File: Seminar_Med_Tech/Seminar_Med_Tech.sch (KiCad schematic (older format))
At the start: 25 parts

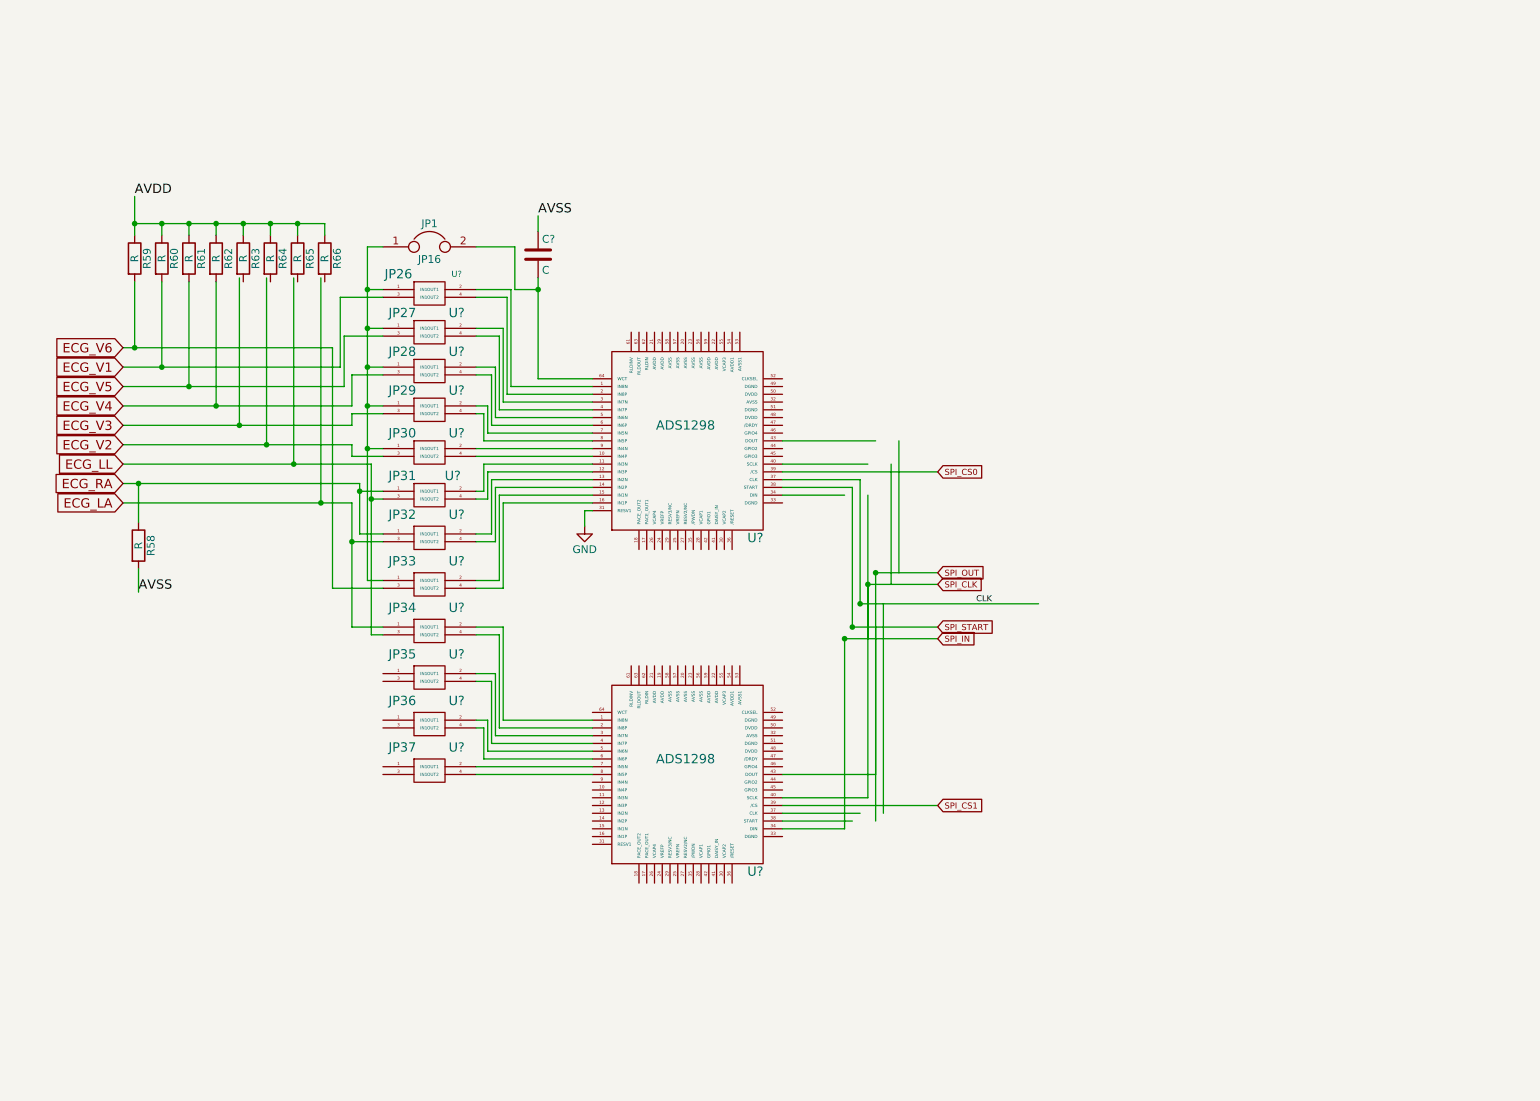
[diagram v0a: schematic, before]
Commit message: Updated Schaltbild
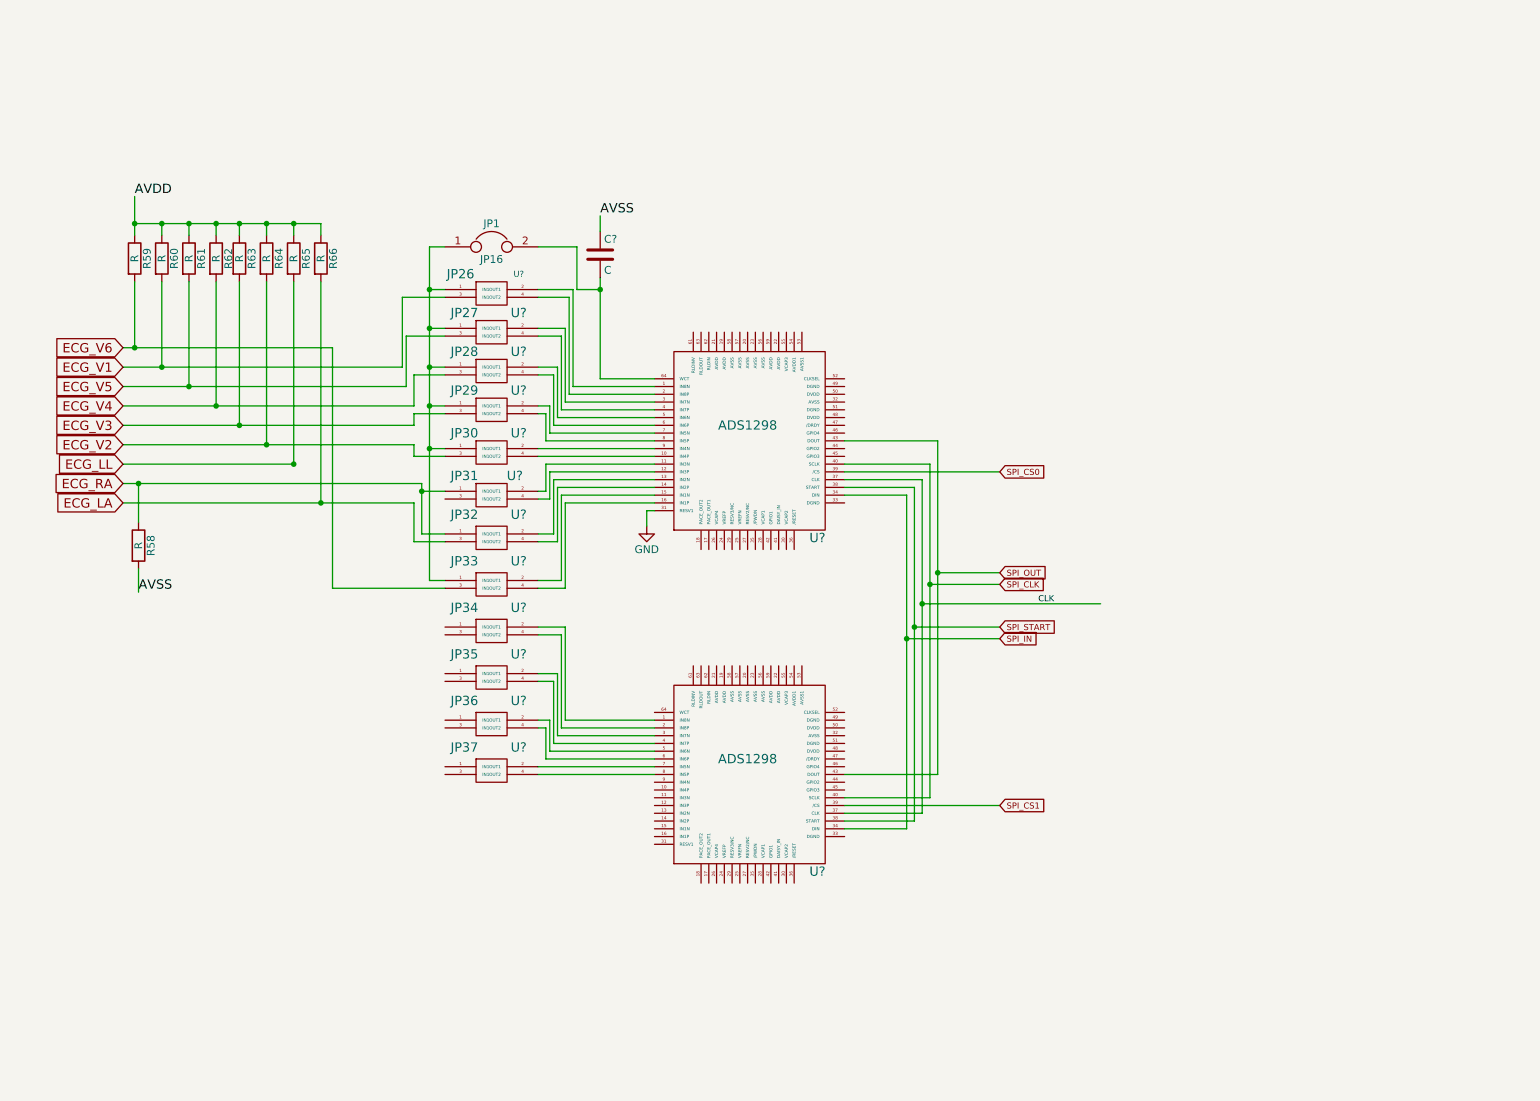
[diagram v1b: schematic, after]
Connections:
- wire segments 156 -> 147
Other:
- moved on the sheet: C?, JP1, R63, R64, R65, R66, U?

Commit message: Updated Schaltbil
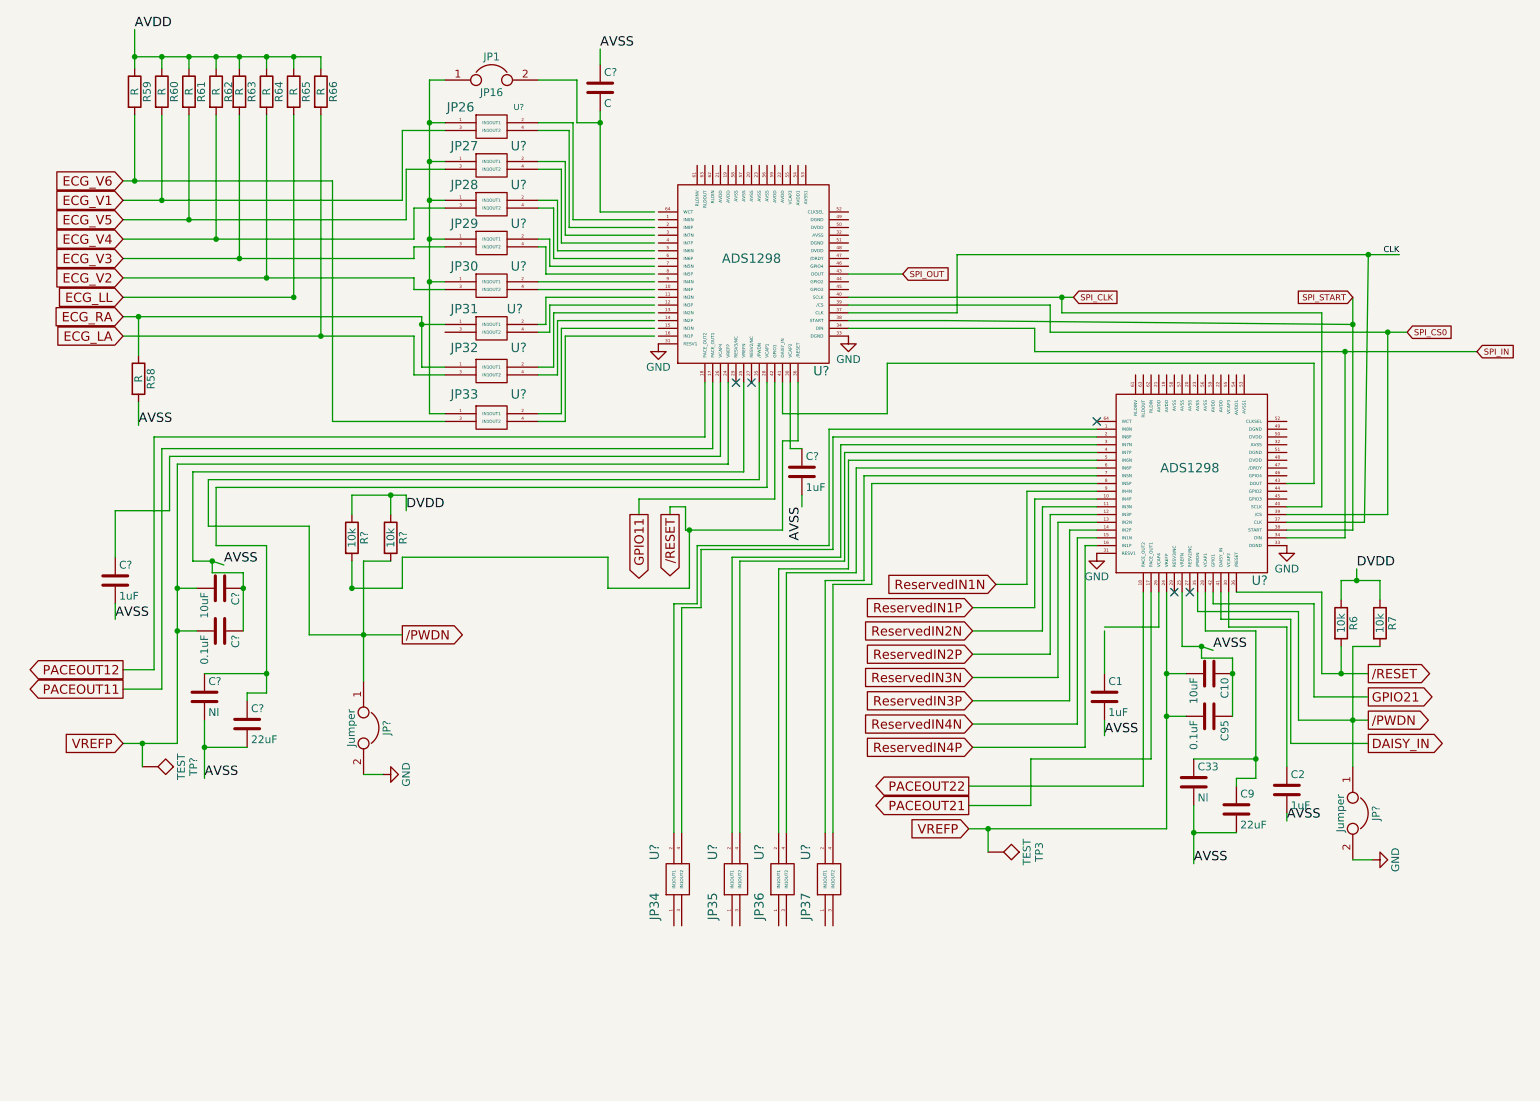
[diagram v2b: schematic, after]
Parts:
- added C1, C2, C? (x2): 1uF, symbol C
- added C10, C?: 10uF, symbol C
- added C33, C?: Nl, symbol C
- added C9, C?: 22uF, symbol C
- added C95, C?: 0.1uF, symbol C
- added JP? (x2): Jumper, symbol Jumper
- added R6, R7, R? (x2): 10k, symbol R
- added TP3, TP?: TEST, symbol TEST
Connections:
- net labels added: /PWDN, /RESET, DAISY_IN, DVDD, GPIO11, GPIO21, PACEOUT11, PACEOUT12, PACEOUT21, PACEOUT22, ReservedIN1N, ReservedIN1P, ReservedIN2N, ReservedIN2P, ReservedIN3N, ReservedIN3P, ReservedIN4N, ReservedIN4P, VREFP
- net labels removed: SPI_CS1
- wire segments 147 -> 369
- no-connect marks 0 -> 5
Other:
- moved on the sheet: C?, JP1, R58, R59, R60, R61, R62, R63, R64, R65, R66, U?

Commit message: Updated Schaltbild
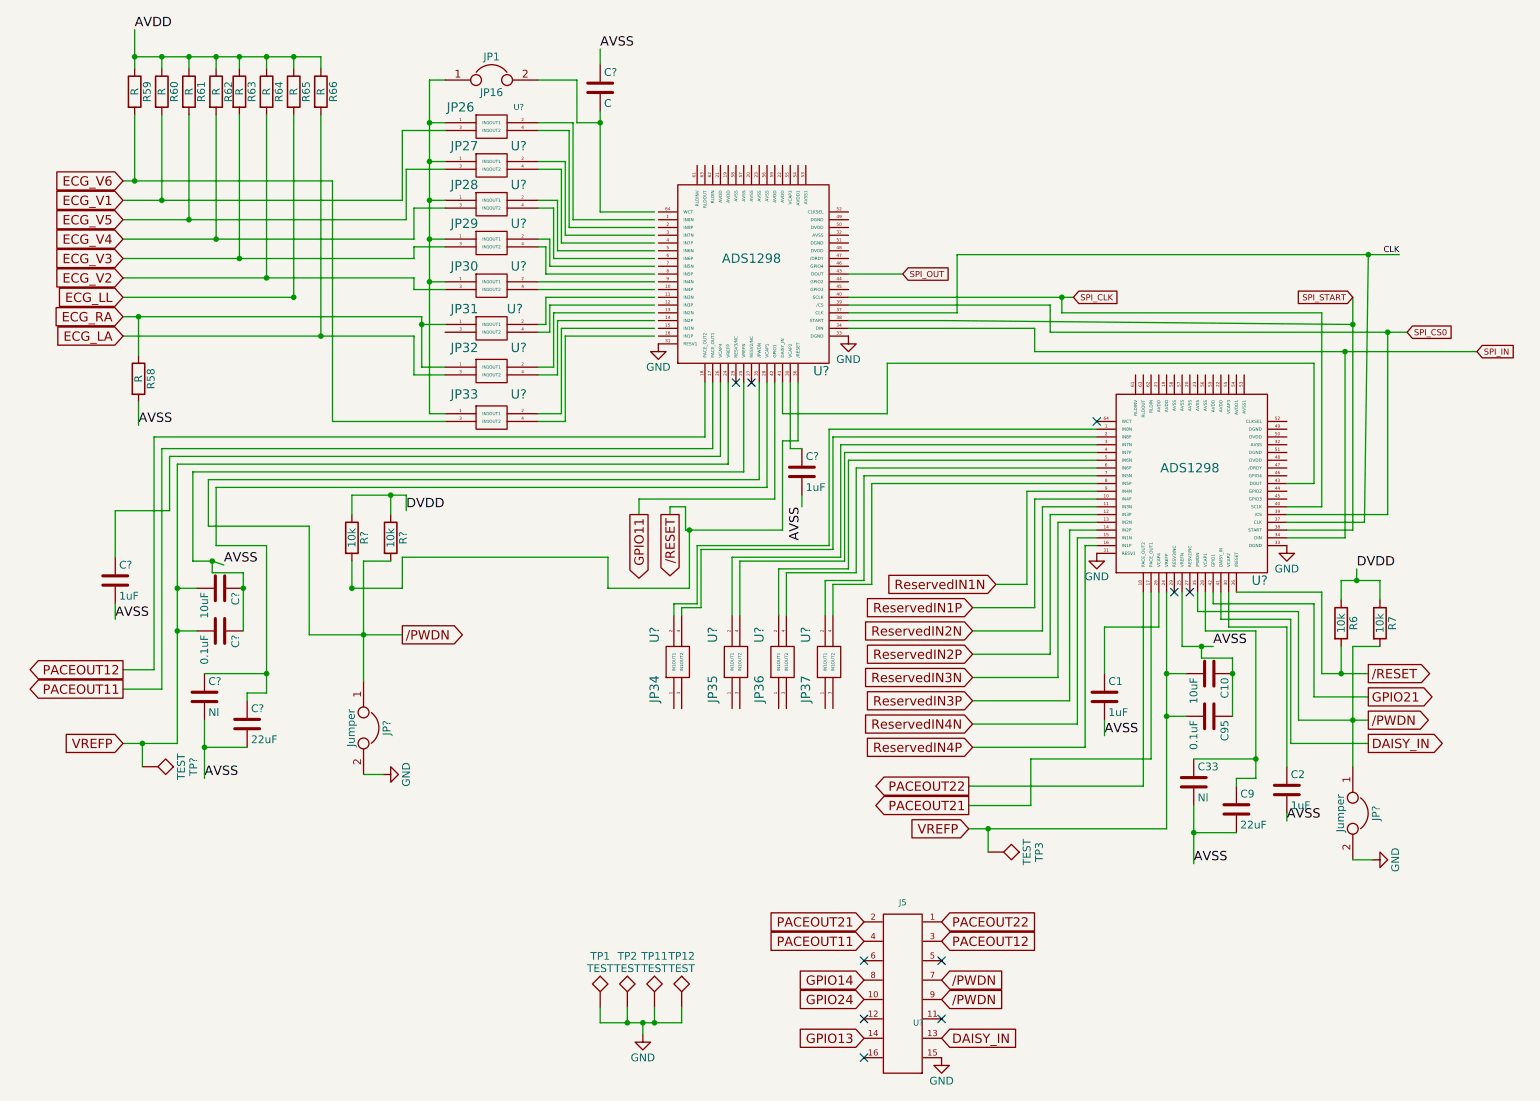
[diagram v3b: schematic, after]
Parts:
- added TP1, TP11, TP12, TP2: TEST, symbol TEST
- added U?: J5, symbol Header12
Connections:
- net labels added: GPIO13, GPIO14, GPIO24
- wire segments 369 -> 327
- no-connect marks 5 -> 10
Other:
- moved on the sheet: U?
